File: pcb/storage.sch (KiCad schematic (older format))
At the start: 11 parts

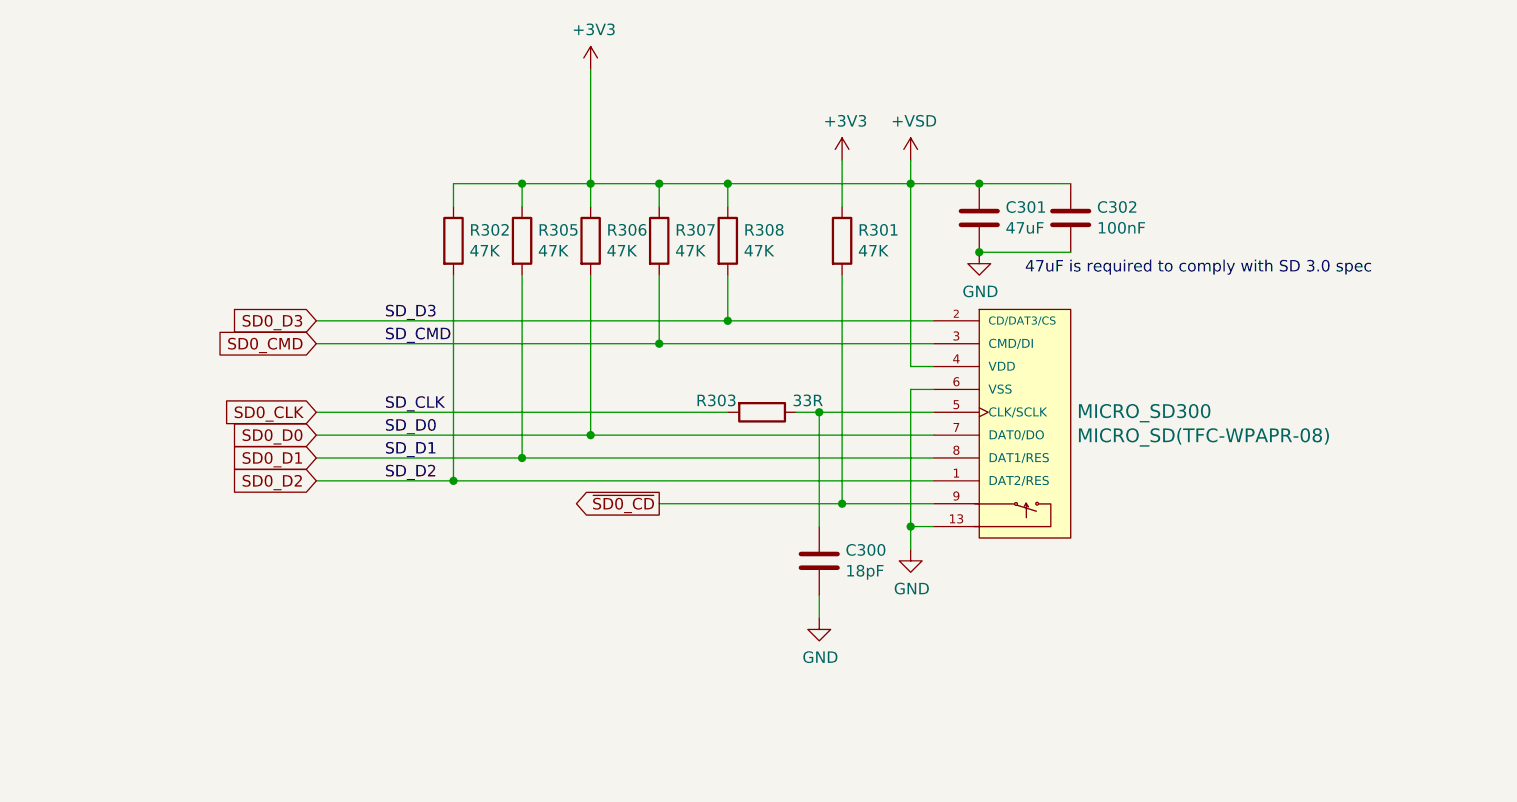
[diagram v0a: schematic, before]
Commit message: sch: working on system config
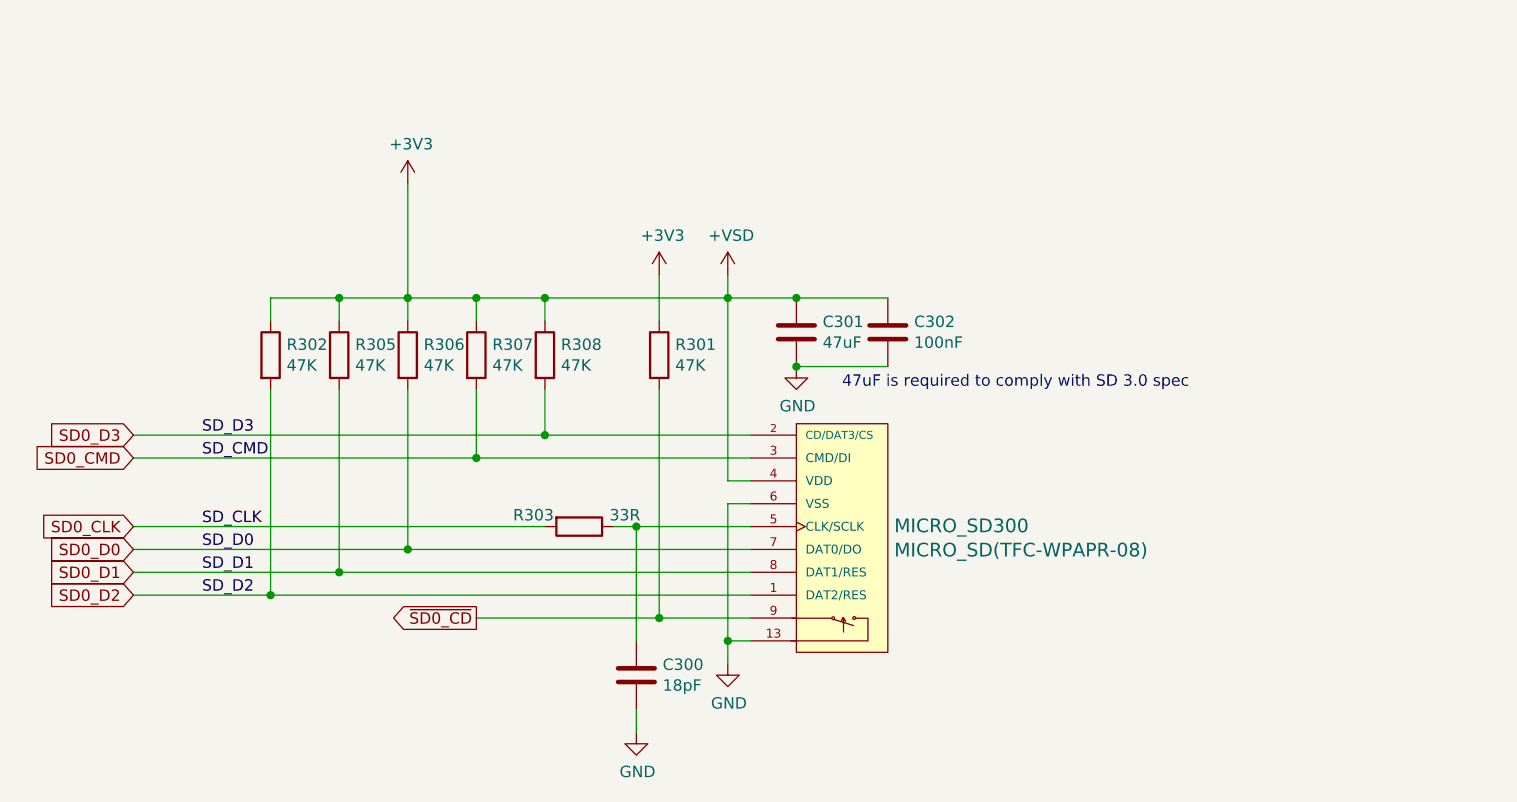
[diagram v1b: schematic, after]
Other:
- moved on the sheet: C300, C301, C302, MICRO_SD300, R301, R302, R303, R305, R306, R307, R308
